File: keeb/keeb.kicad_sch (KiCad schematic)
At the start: 162 parts, among them J101 USB_C_Receptacle_USB2.0, J102 AVR-ISP-6, SW101 SW_Push, SW102 SW_Push, SW103 SW_Push, SW104 SW_Push, SW105 SW_Push, SW106 SW_Push, SW107 SW_Push, SW108 SW_Push, SW109 SW_Push, SW110 SW_Push, SW111 SW_Push, SW112 SW_Push, SW113 SW_Push, SW114 SW_Push, SW115 SW_Push, SW116 SW_Push, SW117 SW_Push, SW118 SW_Push, SW119 SW_Push, SW120 SW_Push, SW121 SW_Push, SW122 SW_Push, SW123 SW_Push, SW124 SW_Push, SW125 SW_Push, SW126 SW_Push, SW127 SW_Push, SW128 SW_Push, SW129 SW_Push, SW130 SW_Push, SW131 SW_Push, SW132 SW_Push, SW133 SW_Push, SW134 SW_Push, SW135 SW_Push, SW136 SW_Push, SW137 SW_Push, SW138 SW_Push, SW139 SW_Push, SW140 SW_Push, SW141 SW_Push, SW142 SW_Push, SW143 SW_Push, SW144 SW_Push, SW145 SW_Push, SW146 SW_Push, SW147 SW_Push, SW148 SW_Push, SW149 SW_Push, SW150 SW_Push, SW151 SW_Push, SW152 SW_Push, SW153 SW_Push, SW154 SW_Push, SW155 SW_Push, SW156 SW_Push, SW157 SW_Push, SW158 SW_Push, SW159 SW_Push, SW160 SW_Push, SW161 SW_Push, SW162 SW_Push, SW163 SW_Push, SW164 SW_Push, SW165 SW_Push, SW166 SW_Push, SW167 SW_Push, U101 TPD2S017, U102 ATmega32U4-AU, Y101 16Mhz

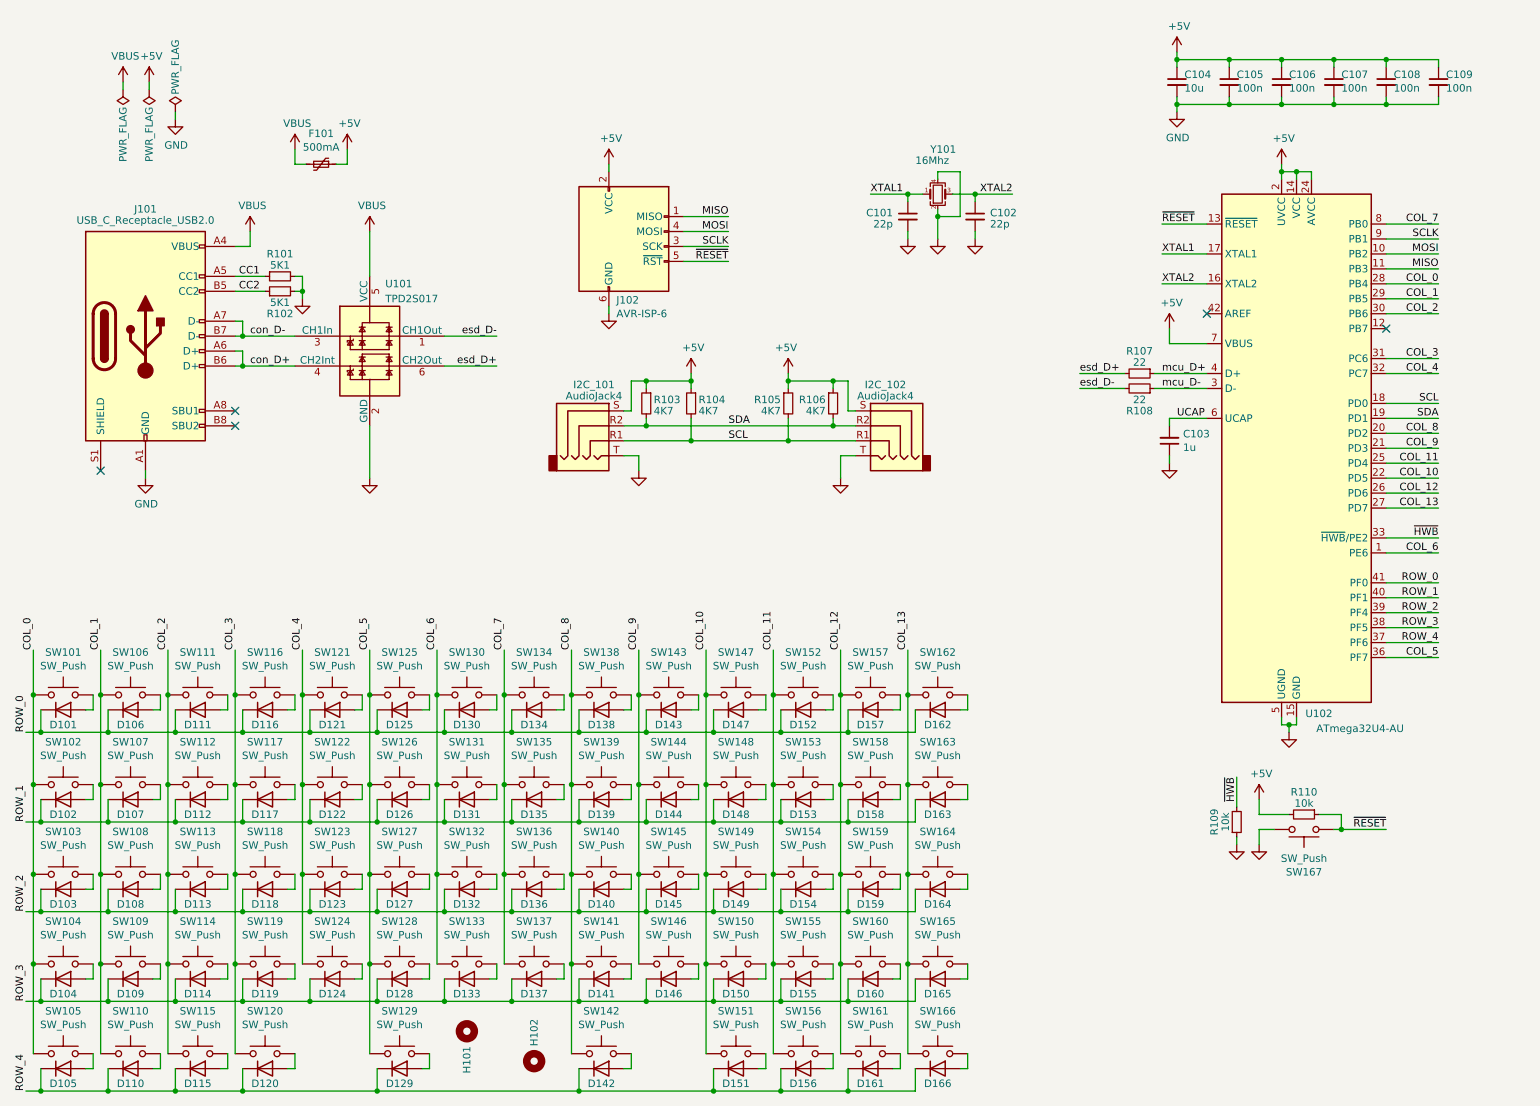
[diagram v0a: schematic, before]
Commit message: footprints, part selection, cleanupo
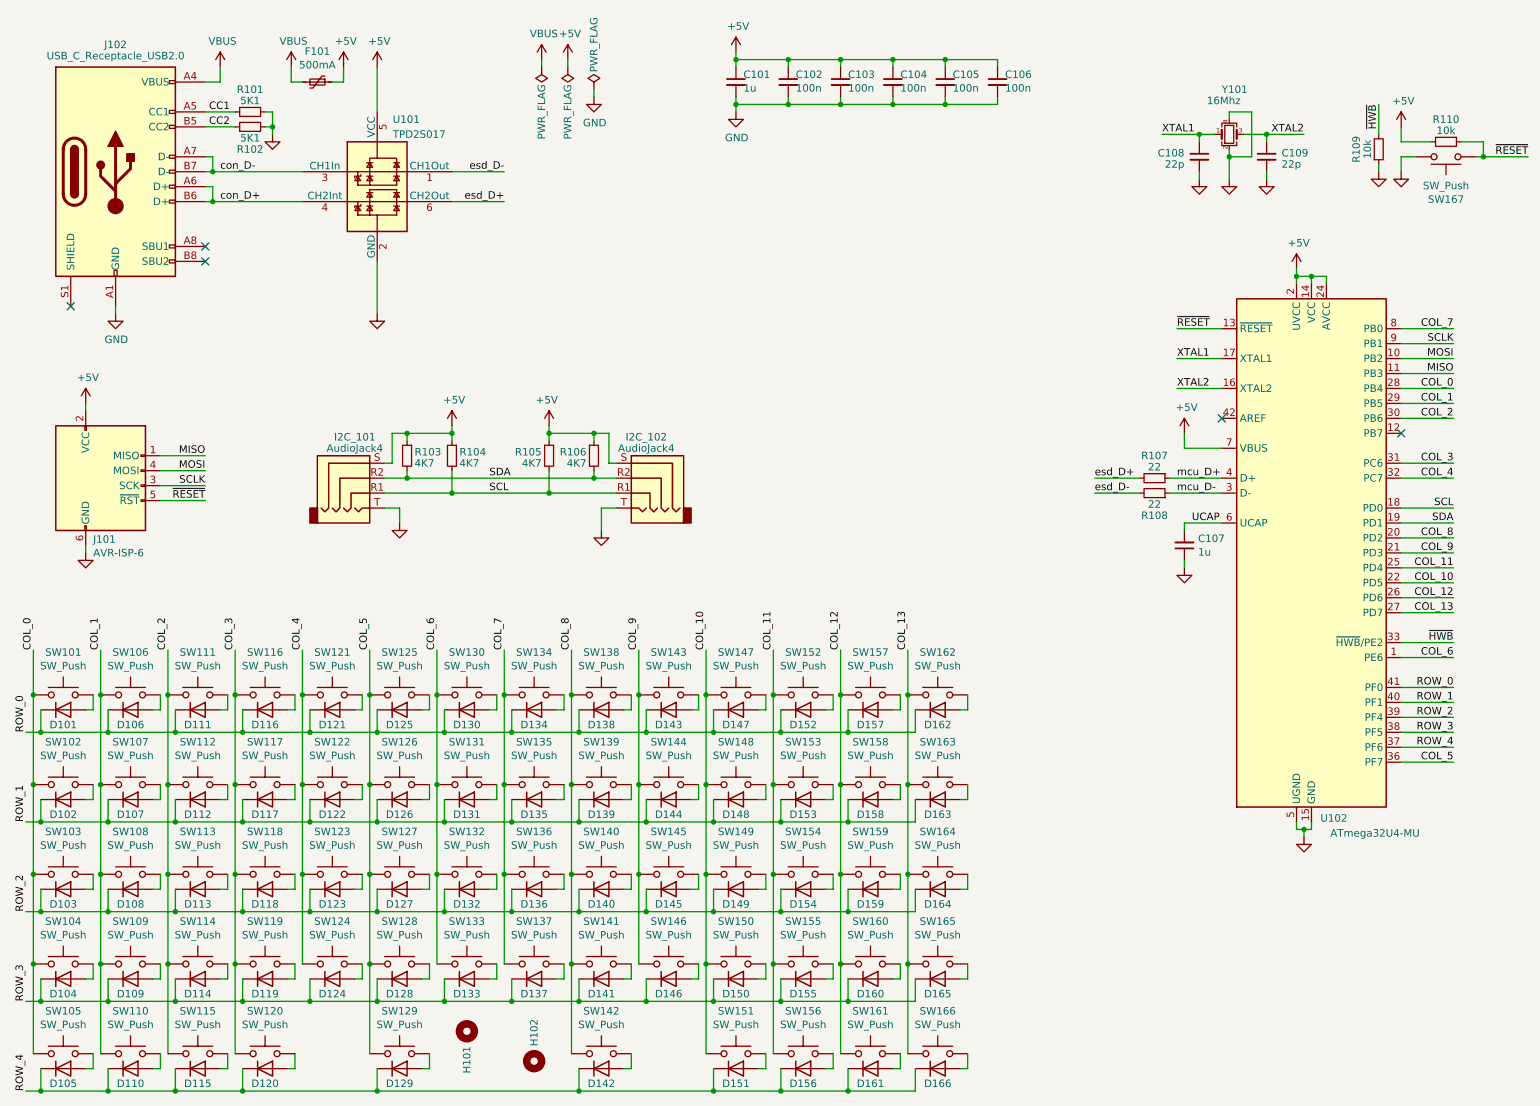
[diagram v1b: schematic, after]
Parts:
- C101: renamed from C104; value 10u -> 1u; footprint Capacitor_SMD:C_1206_3216Metric_Pad1.33x1.80mm_HandSolder -> Capacitor_SMD:C_0603_1608Metric; LCSC # (none) -> C15849; LCSC Link (none) -> https://datasheet.lcsc.com/lcsc/1810261812_Samsung-Electro-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
- C102: renamed from C105; LCSC # (none) -> C1525; LCSC Link (none) -> https://www.lcsc.com/product-detail/Multilayer-Ceramic-Capa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
- C103: renamed from C106; LCSC # (none) -> C1525; LCSC Link (none) -> https://www.lcsc.com/product-detail/Multilayer-Ceramic-Capa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
- C104: renamed from C107; LCSC # (none) -> C1525; LCSC Link (none) -> https://www.lcsc.com/product-detail/Multilayer-Ceramic-Capa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
- C105: renamed from C108; LCSC # (none) -> C1525; LCSC Link (none) -> https://www.lcsc.com/product-detail/Multilayer-Ceramic-Capa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
- C106: renamed from C109; LCSC # (none) -> C1525; LCSC Link (none) -> https://www.lcsc.com/product-detail/Multilayer-Ceramic-Capa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
- C107: renamed from C103; footprint Capacitor_SMD:C_0402_1005Metric -> Capacitor_SMD:C_0603_1608Metric; LCSC # (none) -> C15849; LCSC Link (none) -> https://datasheet.lcsc.com/lcsc/1810261812_Samsung-Electro-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
- D101, D102, D103, D104, D105, D106, D107, D108, D109, D110, D111, D112, D113, D114, D115, D116, D117, D118, D119, D120, D121, D122, D123, D124, D125, D126, D127, D128, D129, D130, D131, D132, D133, D134, D135, D136, D137, D138, D139, D140, D141, D142, D143, D144, D145, D146, D147, D148, D149, D150, D151, D152, D153, D154, D155, D156, D157, D158, D159, D160, D161, D162, D163, D164, D165, D166: footprint Diode_SMD:D_SOD-323F -> Diode_SMD:D_SOD-123F; LCSC # (none) -> C64898; LCSC Link (none) -> https://www.lcsc.com/product-detail/Diodes---General-Purpos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
- F101: footprint Fuse:Fuse_1206_3216Metric_Pad1.42x1.75mm_HandSolder -> Fuse:Fuse_0603_1608Metric; LCSC # (none) -> C369159; LCSC Link (none) -> https://www.lcsc.com/product-detail/Resettable-Fuses_Jinrui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
- I2C_101, I2C_102: LCSC # (none) -> C388632; LCSC Link (none) -> https://www.lcsc.com/product-detail/Audio-Connectors_XKB-Co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; Supplier # digi: 839-54-00177CT-ND -> (none)
- J102: renamed from J101; LCSC # (none) -> C165948; LCSC Link (none) -> https://www.lcsc.com/product-detail/USB-Connectors_Korean-H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; Supplier # LCSC: C165948 -> (none)
- SW167: LCSC # (none) -> C231329; LCSC Link (none) -> https://www.lcsc.com/product-detail/Tactile-Switches_Omron-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; Supplier # LCSC: C231329 -> (none)
- U101: LCSC # (none) -> C880115; LCSC Link (none) -> https://www.lcsc.com/product-detail/ESD-Protection-Devices_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
- U102: value ATmega32U4-AU -> ATmega32U4-MU; LCSC # (none) -> C112161; LCSC Link (none) -> https://www.lcsc.com/product-detail/Microcontroller-Units-M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; Supplier # digi: ATMEGA32U4RC-AU-ND -> (none)
- Y101: LCSC https://www.lcsc.com/product-detail/Crystals_YLFailong-Crys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 -> (none); LCSC # (none) -> C431146; LCSC Link (none) -> https://www.lcsc.com/product-detail/Crystals_YLFailong-Crys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; LCSC# C431146 -> (none)
- renumbered C101 to C108, C102 to C109, J102 to J101
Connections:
- net +5V: now also U101.5 (VCC)
- net VBUS: no longer U101.5 (VCC)
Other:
- moved on the sheet: C101, C102, C103, C104, C105, C106, C107, C108, C109, F101, I2C_101, J101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
